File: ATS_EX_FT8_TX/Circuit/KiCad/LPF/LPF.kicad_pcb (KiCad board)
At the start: 2 copper layers, 84.5 x 23.5 mm, 11 parts

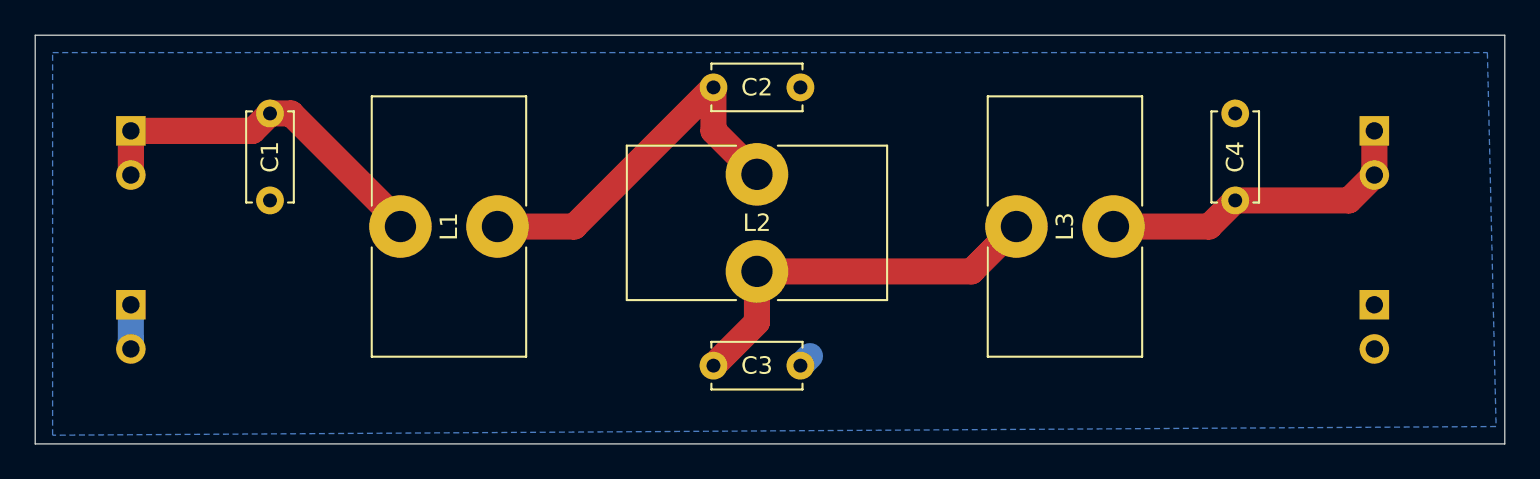
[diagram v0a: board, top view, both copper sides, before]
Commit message: LPF update
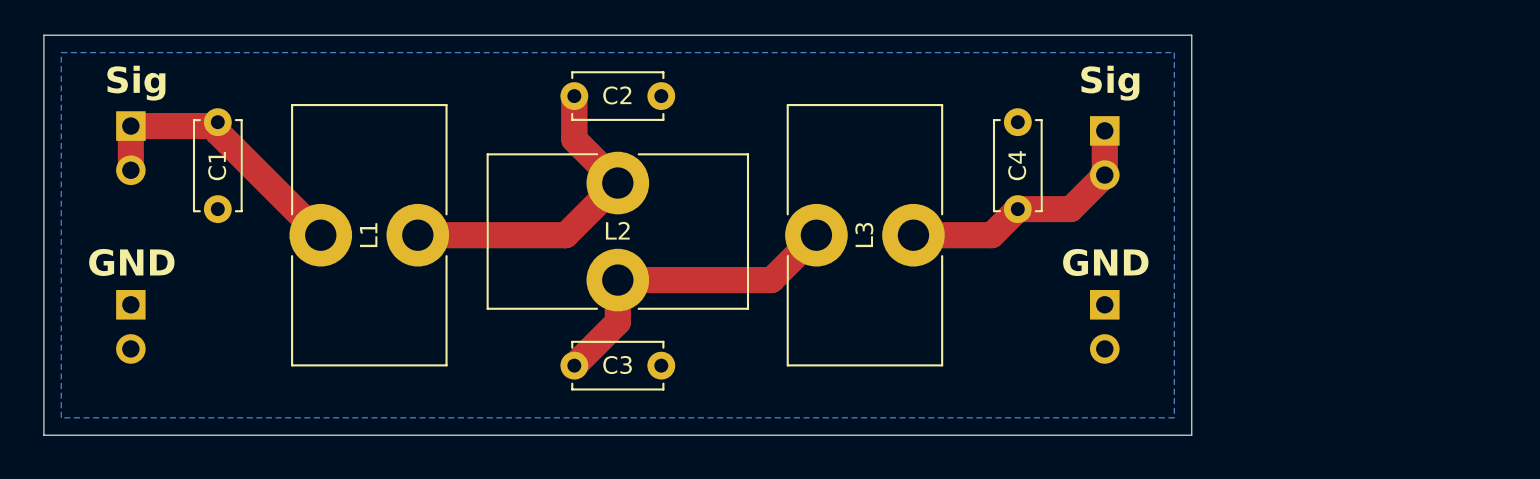
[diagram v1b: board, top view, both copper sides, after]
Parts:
- moved GND 15.5 mm to (129.5, 60.5)
- moved Sig 15.5 mm to (129.5, 50.5)
- moved C4 12.5 mm to (124.5, 55.0)
- moved L3 11.5 mm to (112.9, 56.5)
- moved C2 8.02 mm to (99.0, 48.5)
- moved L2 8.02 mm to (101.5, 53.5)
- moved C3 8.00 mm to (99.0, 64.0)
- moved L1 4.61 mm to (84.4, 56.5)
- moved C1 3.04 mm to (78.5, 50.0)
- moved Sig 0.27 mm to (73.5, 50.2)
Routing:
- net Net-(C1-+): track 21.4 -> 16.6 mm
- net Net-(C3-+): track 22.4 -> 18.4 mm
- net GND: track 3.86 -> 0.00 mm
- net Net-(C4-+): track 18.8 -> 15.0 mm
- net Net-(C2-+): track 21.6 -> 18.8 mm
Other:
- board size 84.5 x 23.5 mm -> 66 x 23 mm
- board text added: "GND"
- board text added: "Sig"
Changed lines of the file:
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@@
 	(footprint "Inductor_THT:L_Toroid_Vertical_L14.7mm_W8.6mm_P5.58mm_Pulse_KM-1"
 		(layer "F.Cu")
-		(at 124.42 56 90)
+		(at 112.92 56.5 90)
 		(descr "L_Toroid, Vertical series, Radial, pin pitch=5.58mm, length*width=14.73*8.64mm^2, Pulse, KM-1, http://datasheet.octopart.com/PE-92112KNL-Pulse-datasheet-17853305.pdf")
 		(tags "L_Toroid Vertical series Radial pin pitch 5.58mm  length 14.73mm width 8.64mm Pulse KM-1")
@@
 	(footprint "Capacitor_THT:C_Disc_D5.0mm_W2.5mm_P5.00mm"
 		(layer "F.Cu")
-		(at 107 64)
+		(at 99 64)
 		(descr "C, Disc series, Radial, pin pitch=5.00mm, diameter*width=5*2.5mm^2, Capacitor, http://cdn-reichelt.de/documents/datenblatt/B300/DS_KERKO_TC.pdf")
 		(tags "C Disc series Radial pin pitch 5.00mm diameter 5mm width 2.5mm Capacitor")
@@
 	(footprint "Inductor_THT:L_Toroid_Vertical_L14.7mm_W8.6mm_P5.58mm_Pulse_KM-1"
 		(layer "F.Cu")
-		(at 109.5 53)
+		(at 101.5 53.5)
 		(descr "L_Toroid, Vertical series, Radial, pin pitch=5.58mm, length*width=14.73*8.64mm^2, Pulse, KM-1, http://datasheet.octopart.com/PE-92112KNL-Pulse-datasheet-17853305.pdf")
 		(tags "L_Toroid Vertical series Radial pin pitch 5.58mm  length 14.73mm width 8.64mm Pulse KM-1")
@@
 	(footprint "Capacitor_THT:C_Disc_D5.0mm_W2.5mm_P5.00mm"
 		(layer "F.Cu")
-		(at 107 48)
+		(at 99 48.5)
 		(descr "C, Disc series, Radial, pin pitch=5.00mm, diameter*width=5*2.5mm^2, Capacitor, http://cdn-reichelt.de/documents/datenblatt/B300/DS_KERKO_TC.pdf")
 		(tags "C Disc series Radial pin pitch 5.00mm diameter 5mm width 2.5mm Capacitor")
@@
 	(footprint "Inductor_THT:L_Toroid_Vertical_L14.7mm_W8.6mm_P5.58mm_Pulse_KM-1"
 		(layer "F.Cu")
-		(at 89 56 90)
+		(at 84.42 56.5 90)
 		(descr "L_Toroid, Vertical series, Radial, pin pitch=5.58mm, length*width=14.73*8.64mm^2, Pulse, KM-1, http://datasheet.octopart.com/PE-92112KNL-Pulse-datasheet-17853305.pdf")
 		(tags "L_Toroid Vertical series Radial pin pitch 5.58mm  length 14.73mm width 8.64mm Pulse KM-1")
@@
 	(footprint "Capacitor_THT:C_Disc_D5.0mm_W2.5mm_P5.00mm"
 		(layer "F.Cu")
-		(at 81.5 49.5 -90)
+		(at 78.5 50 -90)
 		(descr "C, Disc series, Radial, pin pitch=5.00mm, diameter*width=5*2.5mm^2, Capacitor, http://cdn-reichelt.de/documents/datenblatt/B300/DS_KERKO_TC.pdf")
 		(tags "C Disc series Radial pin pitch 5.00mm diameter 5mm width 2.5mm Capacitor")
@@
 	(footprint "Capacitor_THT:C_Disc_D5.0mm_W2.5mm_P5.00mm"
 		(layer "F.Cu")
-		(at 137 54.5 90)
+		(at 124.5 55 90)
 		(descr "C, Disc series, Radial, pin pitch=5.00mm, diameter*width=5*2.5mm^2, Capacitor, http://cdn-reichelt.de/documents/datenblatt/B300/DS_KERKO_TC.pdf")
 		(tags "C Disc series Radial pin pitch 5.00mm diameter 5mm width 2.5mm Capacitor")
@@
 	(footprint "Connector_PinHeader_2.54mm:PinHeader_1x02_P2.54mm_Vertical"
 		(layer "B.Cu")
-		(at 73.5 50.5 180)
+		(at 73.5 50.225 180)
 		(descr "Through hole straight pin header, 1x02, 2.54mm pitch, single row")
 		(tags "Through hole pin header THT 1x02 2.54mm single row")
@@
 	(footprint "Connector_PinHeader_2.54mm:PinHeader_1x02_P2.54mm_Vertical"
 		(layer "B.Cu")
-		(at 145 50.5 180)
+		(at 129.5 50.5 180)
 		(descr "Through hole straight pin header, 1x02, 2.54mm pitch, single row")
 		(tags "Through hole pin header THT 1x02 2.54mm single row")
@@
 	(footprint "Connector_PinHeader_2.54mm:PinHeader_1x02_P2.54mm_Vertical"
 		(layer "B.Cu")
-		(at 145 60.5 180)
+		(at 129.5 60.5 180)
 		(descr "Through hole straight pin header, 1x02, 2.54mm pitch, single row")
 		(tags "Through hole pin header THT 1x02 2.54mm single row")
@@
 			)
 			(layer "B.Fab")
-		)
-		(fp_text user "${REFERENCE}"
-			(at 0 -1.27 90)
-			(layer "B.Fab")
-			(effects
-				(font
-					(size 1 1)
-					(thickness 0.15)
-				)
-				(justify mirror)
-			)
 		)
 		(pad "1" thru_hole rect
@@
 	)
 	(gr_rect
-		(start 68 45)
-		(end 152.5 68.5)
+		(start 68.5 45)
+		(end 134.5 68)
 		(stroke
 			(width 0.05)
@@
 		(layer "Edge.Cuts")
 	)
+	(gr_text "Sig"
+		(at 128 48.5 0)
+		(layer "F.SilkS")
+		(effects
+			(font
+				(size 1.5 1.5)
+				(thickness 0.3)
+				(bold yes)
+			)
+			(justify left bottom)
+		)
+	)
+	(gr_text "GND"
+		(at 127 59 0)
+		(layer "F.SilkS")
+		(effects
+			(font
+				(size 1.5 1.5)
+				(thickness 0.3)
+				(bold yes)
+			)
+			(justify left bottom)
+		)
+	)
+	(gr_text "GND"
+		(at 71 59 0)
+		(layer "F.SilkS")
+		(effects
+			(font
+				(size 1.5 1.5)
+				(thickness 0.3)
+				(bold yes)
+			)
+			(justify left bottom)
+		)
+	)
+	(gr_text "Sig"
+		(at 72 48.5 0)
+		(layer "F.SilkS")
+		(effects
+			(font
+				(size 1.5 1.5)
+				(thickness 0.3)
+				(bold yes)
+			)
+			(justify left bottom)
+		)
+	)
 	(segment
-		(start 73.5 63.04)
-		(end 73.5 62.5)
-		(width 1.5)
-		(layer "B.Cu")
-		(net 1)
-	)
-	(segment
-		(start 112 64)
-		(end 112.551 63.449)
-		(width 1.5)
-		(layer "B.Cu")
-		(net 1)
-	)
-	(segment
-		(start 73.5 60.5)
-		(end 73.5 63.04)
-		(width 1.5)
-		(layer "B.Cu")
-		(net 1)
-	)
-	(segment
-		(start 80.5 50.5)
-		(end 81.5 49.5)
+		(start 78.275 50.225)
+		(end 78.5 50)
 		(width 1.5)
 		(layer "F.Cu")
@@
 	)
 	(segment
-		(start 82.71 49.5)
-		(end 89.21 56)
+		(start 78.5 50.58)
+		(end 84.42 56.5)
 		(width 1.5)
 		(layer "F.Cu")
@@
 	)
 	(segment
-		(start 81.5 49.5)
-		(end 82.71 49.5)
+		(start 73.5 52.765)
+		(end 73.5 50.225)
 		(width 1.5)
 		(layer "F.Cu")
@@
 	)
 	(segment
-		(start 73.5 53.04)
-		(end 73.5 50.5)
+		(start 73.5 50.225)
+		(end 78.275 50.225)
 		(width 1.5)
 		(layer "F.Cu")
@@
 	)
 	(segment
-		(start 73.5 50.5)
-		(end 80.5 50.5)
+		(start 78.5 50)
+		(end 78.5 50.58)
 		(width 1.5)
 		(layer "F.Cu")
@@
 	)
 	(segment
-		(start 107 50.5)
-		(end 109.5 53)
+		(start 90 56.5)
+		(end 98.5 56.5)
 		(width 1.5)
 		(layer "F.Cu")
@@
 	)
 	(segment
-		(start 107 48)
-		(end 107 50.5)
+		(start 98.5 56.5)
+		(end 101.5 53.5)
 		(width 1.5)
 		(layer "F.Cu")
@@
 	)
 	(segment
-		(start 99 56)
-		(end 107 48)
+		(start 99 51)
+		(end 101.5 53.5)
 		(width 1.5)
 		(layer "F.Cu")
@@
 	)
 	(segment
-		(start 94.79 56)
-		(end 99 56)
+		(start 99 48.5)
+		(end 99 51)
 		(width 1.5)
 		(layer "F.Cu")
@@
 	)
 	(segment
-		(start 121.84 58.58)
-		(end 124.42 56)
+		(start 101.5 59.08)
+		(end 101.5 61.5)
 		(width 1.5)
 		(layer "F.Cu")
@@
 	)
 	(segment
-		(start 109.5 58.58)
-		(end 109.5 61.5)
+		(start 101.5 59.08)
+		(end 110.34 59.08)
 		(width 1.5)
 		(layer "F.Cu")
@@
 	)
 	(segment
-		(start 109.5 61.5)
-		(end 107 64)
+		(start 101.5 61.5)
+		(end 99 64)
 		(width 1.5)
 		(layer "F.Cu")
@@
 	)
 	(segment
-		(start 109.5 58.58)
-		(end 121.84 58.58)
+		(start 110.34 59.08)
+		(end 112.92 56.5)
 		(width 1.5)
 		(layer "F.Cu")
@@
 	)
 	(segment
-		(start 145 53.04)
-		(end 145 50.5)
+		(start 129.5 53.04)
+		(end 129.5 50.5)
 		(width 1.5)
 		(layer "F.Cu")
@@
 	)
 	(segment
-		(start 130 56)
-		(end 135.5 56)
+		(start 124.5 55)
+		(end 127.54 55)
 		(width 1.5)
 		(layer "F.Cu")
@@
 	)
 	(segment
-		(start 143.54 54.5)
-		(end 145 53.04)
+		(start 118.5 56.5)
+		(end 123 56.5)
 		(width 1.5)
 		(layer "F.Cu")
@@
 	)
 	(segment
-		(start 135.5 56)
-		(end 137 54.5)
+		(start 127.54 55)
+		(end 129.5 53.04)
 		(width 1.5)
 		(layer "F.Cu")
@@
 	)
 	(segment
-		(start 137 54.5)
-		(end 143.54 54.5)
+		(start 123 56.5)
+		(end 124.5 55)
 		(width 1.5)
 		(layer "F.Cu")
@@
 		(polygon
 			(pts
-				(xy 69 46) (xy 151.5 46) (xy 152 67.5) (xy 69 68)
-			)
-		)
+				(xy 69.5 46) (xy 133.5 46) (xy 133.5 67) (xy 69.5 67)
+			)
+		)
